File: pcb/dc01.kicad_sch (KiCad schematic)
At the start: 83 parts, among them J1 USB_C_Receptacle_USB2.0, J10 Conn_01x02, J2 PROG/DEBUG, J3 Conn_01x06, J4 RJ12, J5 RJ12, J6 Conn_01x02, J7 Conn_01x02, J8 Conn_01x02, J9 Conn_01x02, K1 AZ850-5, K2 AZ850-5, Q1 2N7002, Q2 2N7002, SW1 SW_Push, SW2 SW_Push, SW3 MFP 113 D, U1 STM32F103C8Tx, U2 AMS1117-3.3, U3 PC817, U4 PC817, Y1 8 MHz

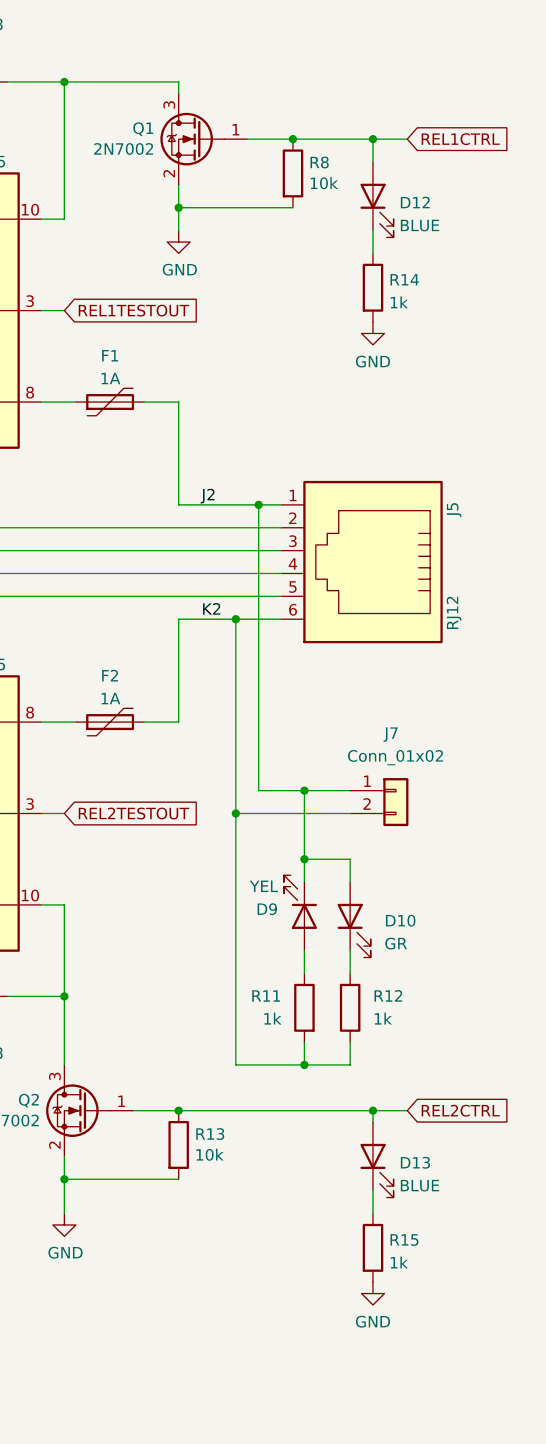
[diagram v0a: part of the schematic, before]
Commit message: Switch relay indication LEDs & resistors.
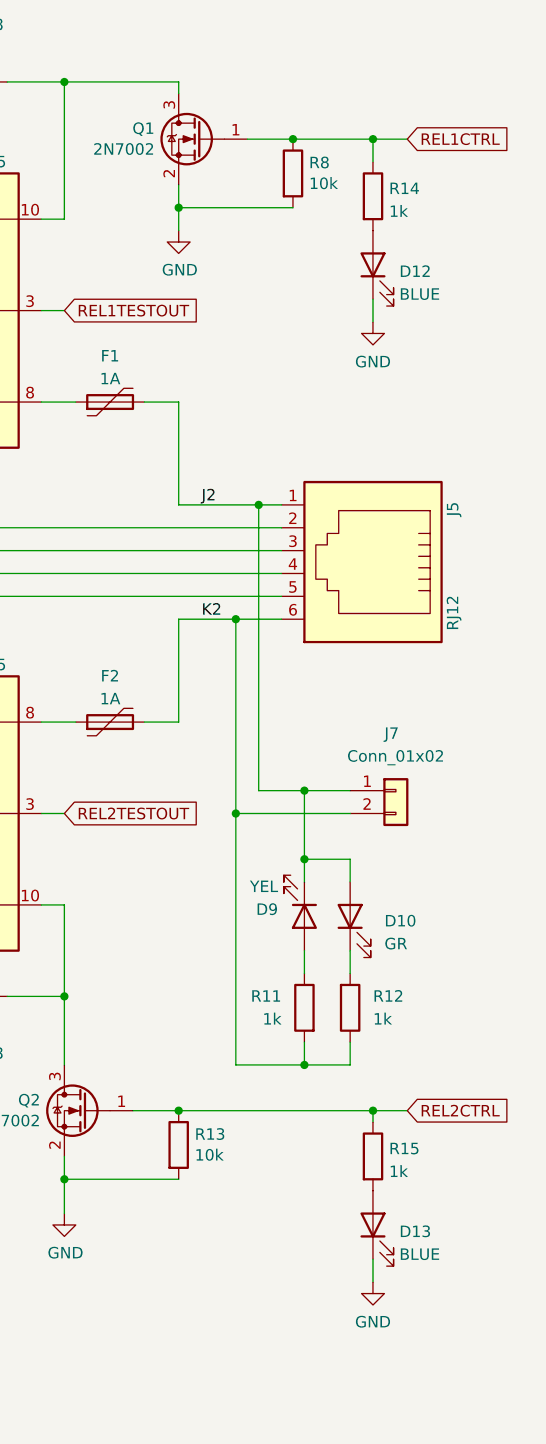
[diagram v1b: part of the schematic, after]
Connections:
- net GND: now also D12.1 (K), D13.1 (K); no longer R14.2, R15.2
- net REL1CTRL: now also R14.1; no longer D12.2 (A)
- net REL2CTRL: now also R15.1; no longer D13.2 (A)
- new net: D13.2 (A), R15.2
- new net: D12.2 (A), R14.2
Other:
- moved on the sheet: D12, D13, R14, R15
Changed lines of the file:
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@@
     (stroke (width 0) (type default) (color 0 0 0 0))
   )
-  (wire (pts (xy 266.7 147.32) (xy 266.7 149.86))
+  (wire (pts (xy 266.7 154.94) (xy 266.7 157.48))
     (stroke (width 0) (type default) (color 0 0 0 0))
   )
@@
     (stroke (width 0) (type default) (color 0 0 0 0))
   )
-  (wire (pts (xy 266.7 40.64) (xy 266.7 43.18))
+  (wire (pts (xy 266.7 48.26) (xy 266.7 50.8))
     (stroke (width 0) (type default) (color 0 0 0 0))
   )
@@
     (pin "2")
   )
-  (symbol (lib_id "Device:R") (at 266.7 153.67 0) (unit 1)
+  (symbol (lib_id "Device:R") (at 266.7 143.51 0) (unit 1)
     (in_bom yes) (on_board yes) (fields_autoplaced)
-    (property "Reference" "R15" (id 0) (at 268.478 152.8353 0)
+    (property "Reference" "R15" (id 0) (at 268.478 142.6753 0)
       (effects (font (size 1.27 1.27)) (justify left))
     )
-    (property "Value" "1k" (id 1) (at 268.478 155.3722 0)
+    (property "Value" "1k" (id 1) (at 268.478 145.2122 0)
       (effects (font (size 1.27 1.27)) (justify left))
     )
-    (property "Footprint" "Resistor_SMD:R_0805_2012Metric" (id 2) (at 264.922 153.67 90)
+    (property "Footprint" "Resistor_SMD:R_0805_2012Metric" (id 2) (at 264.922 143.51 90)
       (effects (font (size 1.27 1.27)) hide)
     )
-    (property "Datasheet" "~" (id 3) (at 266.7 153.67 0)
+    (property "Datasheet" "~" (id 3) (at 266.7 143.51 0)
       (effects (font (size 1.27 1.27)) hide)
     )
@@
     (pin "2")
   )
-  (symbol (lib_id "Device:R") (at 266.7 46.99 0) (unit 1)
+  (symbol (lib_id "Device:R") (at 266.7 36.83 0) (unit 1)
     (in_bom yes) (on_board yes) (fields_autoplaced)
-    (property "Reference" "R14" (id 0) (at 268.478 46.1553 0)
+    (property "Reference" "R14" (id 0) (at 268.478 35.9953 0)
       (effects (font (size 1.27 1.27)) (justify left))
     )
-    (property "Value" "1k" (id 1) (at 268.478 48.6922 0)
+    (property "Value" "1k" (id 1) (at 268.478 38.5322 0)
       (effects (font (size 1.27 1.27)) (justify left))
     )
-    (property "Footprint" "Resistor_SMD:R_0805_2012Metric" (id 2) (at 264.922 46.99 90)
+    (property "Footprint" "Resistor_SMD:R_0805_2012Metric" (id 2) (at 264.922 36.83 90)
       (effects (font (size 1.27 1.27)) hide)
     )
-    (property "Datasheet" "~" (id 3) (at 266.7 46.99 0)
+    (property "Datasheet" "~" (id 3) (at 266.7 36.83 0)
       (effects (font (size 1.27 1.27)) hide)
     )
@@
     (pin "2")
   )
-  (symbol (lib_id "Device:LED") (at 266.7 36.83 90) (unit 1)
+  (symbol (lib_id "Device:LED") (at 266.7 44.45 90) (unit 1)
     (in_bom yes) (on_board yes) (fields_autoplaced)
-    (property "Reference" "D12" (id 0) (at 269.621 37.5828 90)
+    (property "Reference" "D12" (id 0) (at 269.621 45.2028 90)
       (effects (font (size 1.27 1.27)) (justify right))
     )
-    (property "Value" "BLUE" (id 1) (at 269.621 40.1197 90)
+    (property "Value" "BLUE" (id 1) (at 269.621 47.7397 90)
       (effects (font (size 1.27 1.27)) (justify right))
     )
-    (property "Footprint" "LED_SMD:LED_0805_2012Metric" (id 2) (at 266.7 36.83 0)
+    (property "Footprint" "LED_SMD:LED_0805_2012Metric" (id 2) (at 266.7 44.45 0)
       (effects (font (size 1.27 1.27)) hide)
     )
-    (property "Datasheet" "~" (id 3) (at 266.7 36.83 0)
+    (property "Datasheet" "~" (id 3) (at 266.7 44.45 0)
       (effects (font (size 1.27 1.27)) hide)
     )
@@
     (pin "3")
   )
-  (symbol (lib_id "Device:LED") (at 266.7 143.51 90) (unit 1)
+  (symbol (lib_id "Device:LED") (at 266.7 151.13 90) (unit 1)
     (in_bom yes) (on_board yes) (fields_autoplaced)
-    (property "Reference" "D13" (id 0) (at 269.621 144.2628 90)
+    (property "Reference" "D13" (id 0) (at 269.621 151.8828 90)
       (effects (font (size 1.27 1.27)) (justify right))
     )
-    (property "Value" "BLUE" (id 1) (at 269.621 146.7997 90)
+    (property "Value" "BLUE" (id 1) (at 269.621 154.4197 90)
       (effects (font (size 1.27 1.27)) (justify right))
     )
-    (property "Footprint" "LED_SMD:LED_0805_2012Metric" (id 2) (at 266.7 143.51 0)
+    (property "Footprint" "LED_SMD:LED_0805_2012Metric" (id 2) (at 266.7 151.13 0)
       (effects (font (size 1.27 1.27)) hide)
     )
-    (property "Datasheet" "~" (id 3) (at 266.7 143.51 0)
+    (property "Datasheet" "~" (id 3) (at 266.7 151.13 0)
       (effects (font (size 1.27 1.27)) hide)
     )

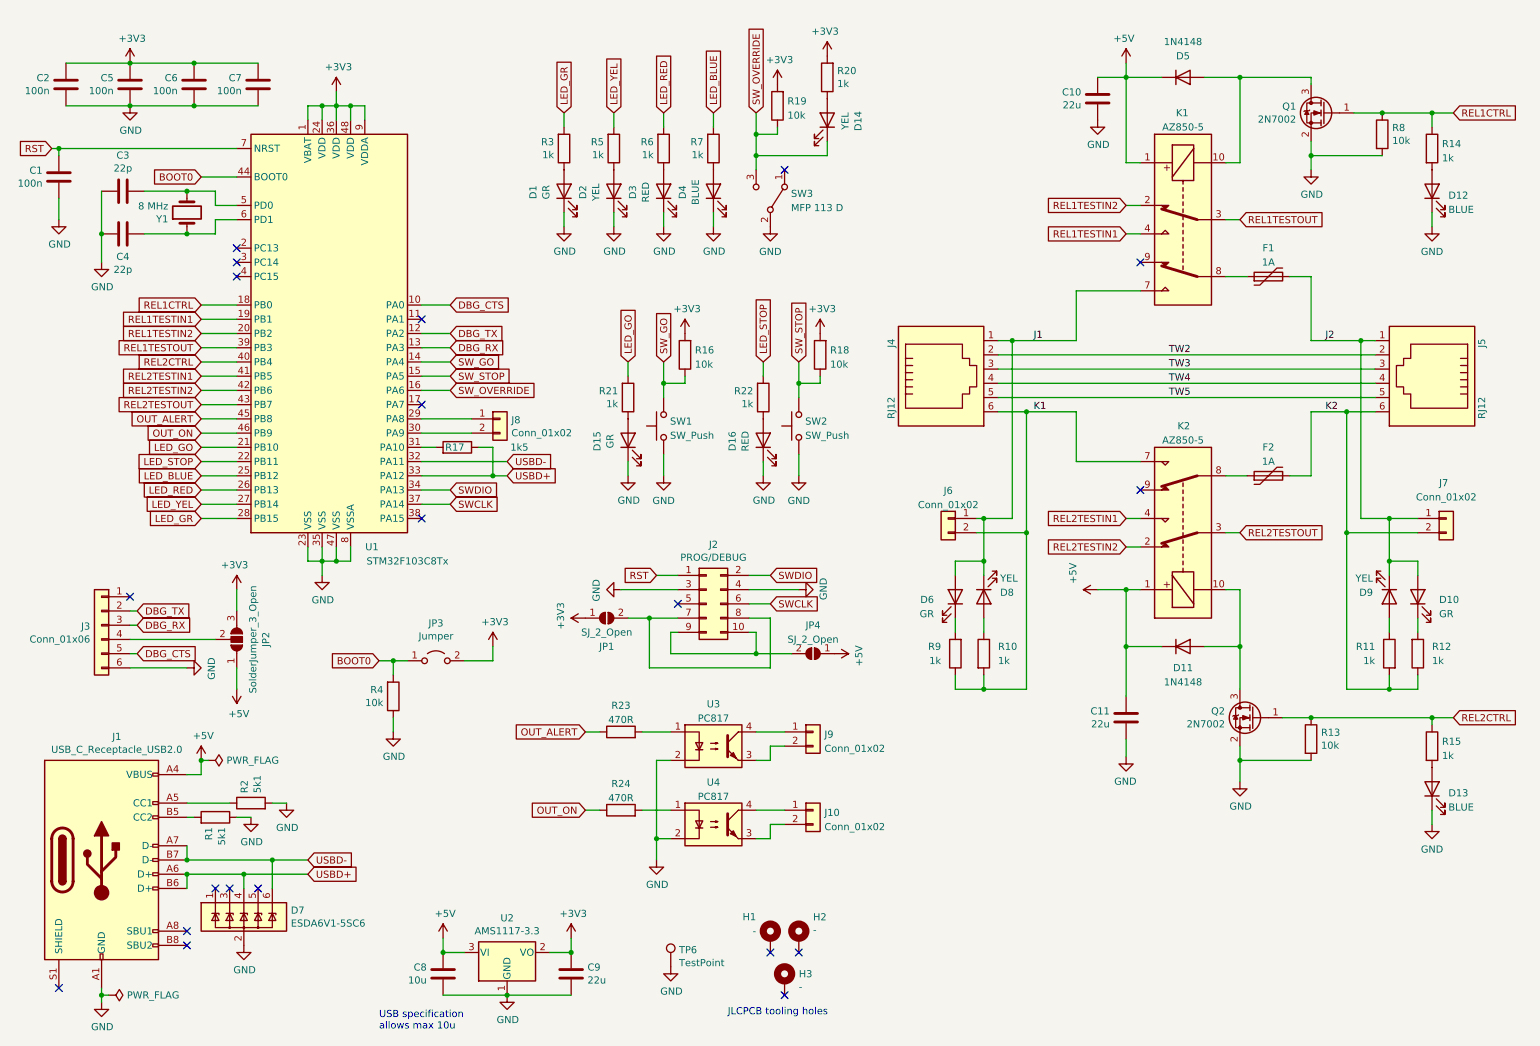
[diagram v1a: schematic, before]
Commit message: Divide into more sheets. Use relays in series.
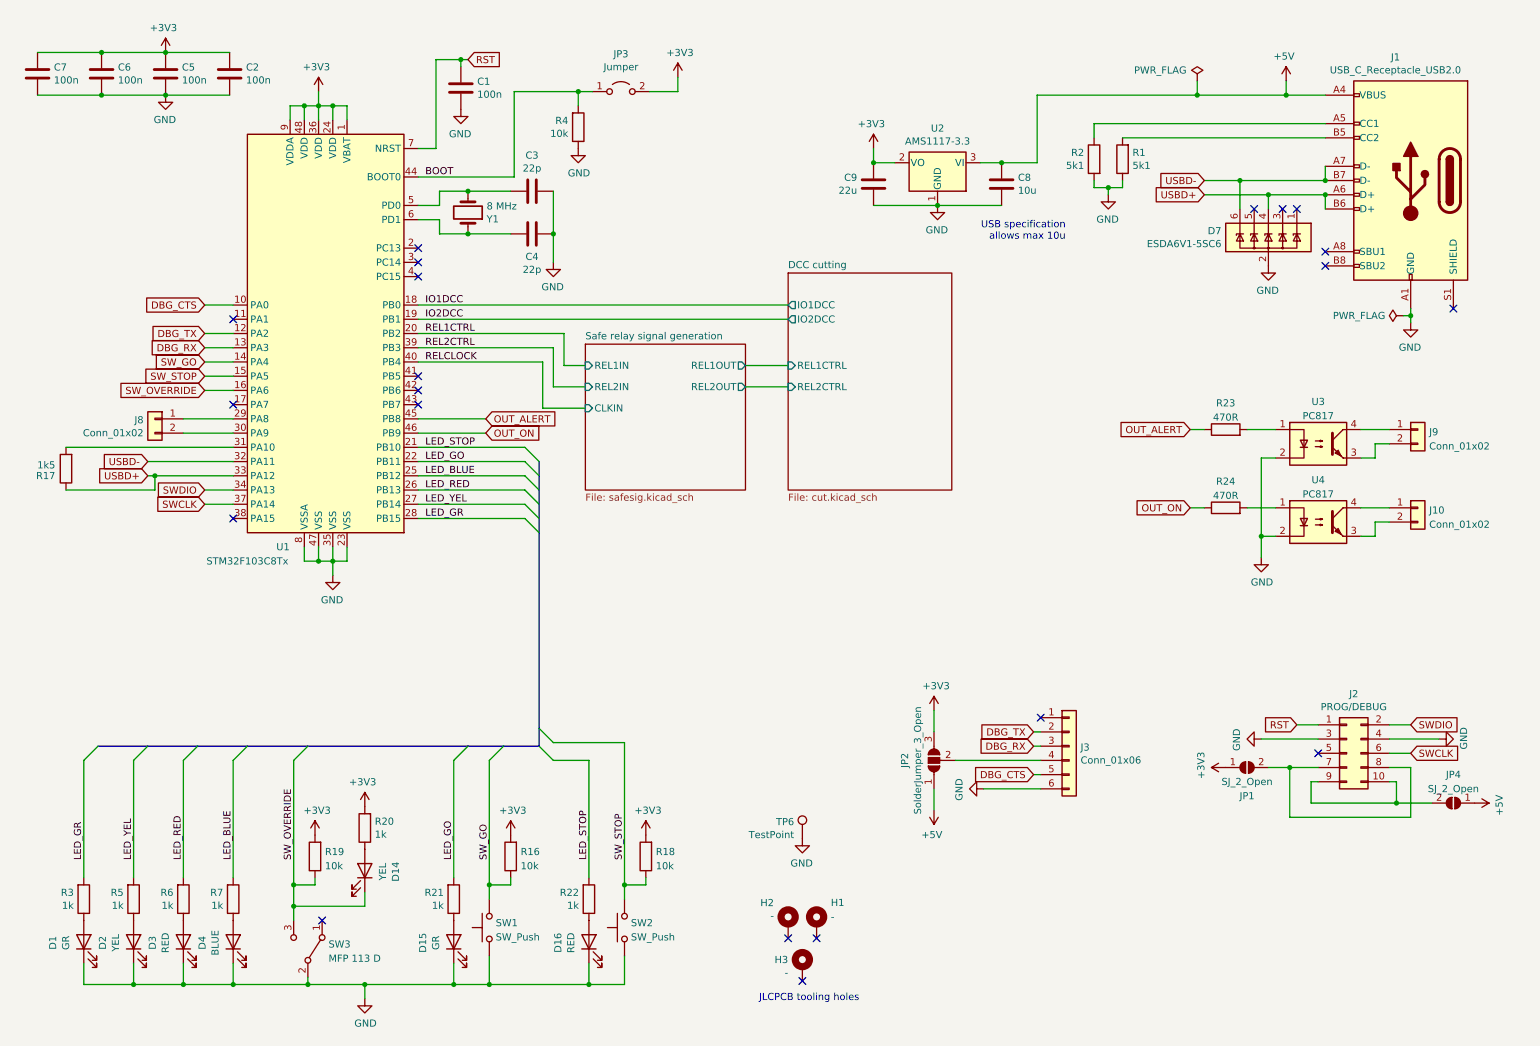
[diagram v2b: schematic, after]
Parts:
- removed C10, C11: 22u, Capacitor_SMD:C_0805_2012Metric, symbol Device:C
- removed D10, D6: GR, LED_SMD:LED_0805_2012Metric, symbol Device:LED
- removed D11, D5: 1N4148, Diode_THT:D_DO-35_SOD27_P7.62mm_Horizontal, symbol Diode:1N4148
- removed D12, D13: BLUE, LED_SMD:LED_0805_2012Metric, symbol Device:LED
- removed D8, D9: YEL, LED_SMD:LED_0805_2012Metric, symbol Device:LED
- removed F1, F2: 1A, Fuse:Fuse_1206_3216Metric, symbol Device:Polyfuse
- removed J4, J5: RJ12, Connector_RJ:RJ25_Wayconn_MJEA-660X1_Horizontal, symbol Connector:RJ12
- removed J6, J7: Conn_01x02, TerminalBlock_Euroclamp:MVE252-5-V, symbol Connector_Generic:Conn_01x02
- removed K1, K2: AZ850-5, Relay_THT:Relay_DPDT_FRT5, symbol Relay:AZ850-x
- removed Q1, Q2: 2N7002, Package_TO_SOT_SMD:SOT-23, symbol Transistor_FET:2N7002
- removed R10, R11, R12, R14, R15, R9: 1k, Resistor_SMD:R_0805_2012Metric, symbol Device:R
- removed R13, R8: 10k, Resistor_SMD:R_0805_2012Metric_Pad1.20x1.40mm_HandSolder, symbol Device:R
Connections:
- net REL1TESTIN2 is gone; now on net REL1CTRL: U1.20 (PB2)
- net REL1TESTOUT is gone; now on net REL2CTRL: U1.39 (PB3)
- net LED_GO: now also U1.22 (PB11); no longer U1.21 (PB10)
- net LED_STOP: now also U1.21 (PB10); no longer U1.22 (PB11)
- net REL1CTRL: no longer U1.18 (PB0)
- net REL2CTRL: no longer U1.40 (PB4)
- net BOOT0 renamed BOOT
- net REL1TESTIN1 renamed IO2DCC
- net REL2TESTIN1: no longer names the net of U1.41 (PB5)
- net REL2TESTIN2: no longer names the net of U1.42 (PB6)
- net REL2TESTOUT: no longer names the net of U1.43 (PB7)
- new net IO1DCC: U1.18 (PB0)
- new net RELCLOCK: U1.40 (PB4)
- no-connect marks 20 -> 21
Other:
- added sheet DCC cutting (cut.kicad_sch)
- added sheet Safe relay signal generation (safesig.kicad_sch)
- title: DCC cutter DC-01 -> DCC cutter DC-01 - overall schematics
- moved on the sheet: C1, C2, C3, C4, C5, C6, C7, C8, C9, D1, D14, D15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
